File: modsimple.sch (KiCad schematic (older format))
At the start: 13 parts, among them J1 MICROUSB, P1 CONN_10, Q2 FDD8870, U1 MAX1555

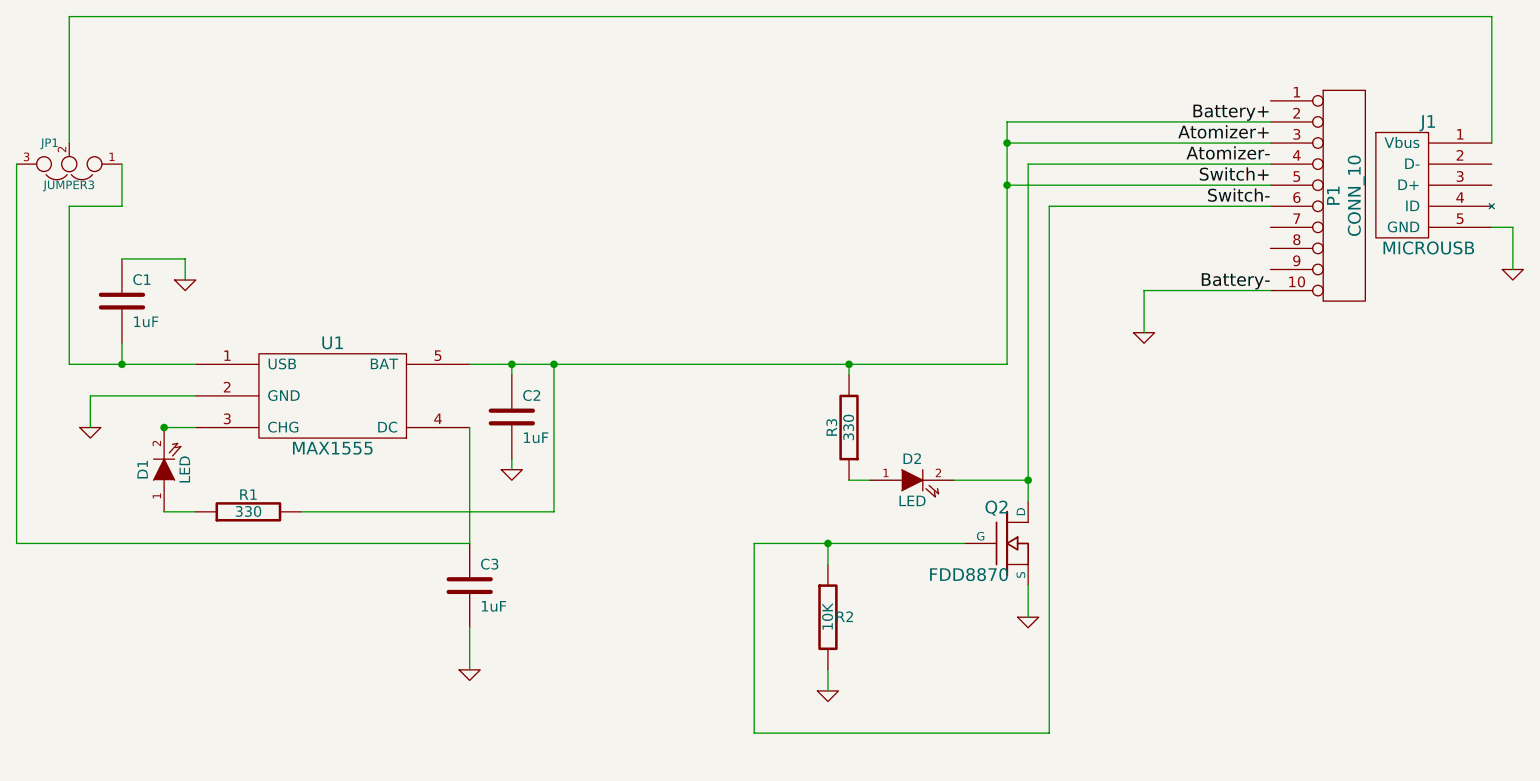
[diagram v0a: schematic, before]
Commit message: cleanup
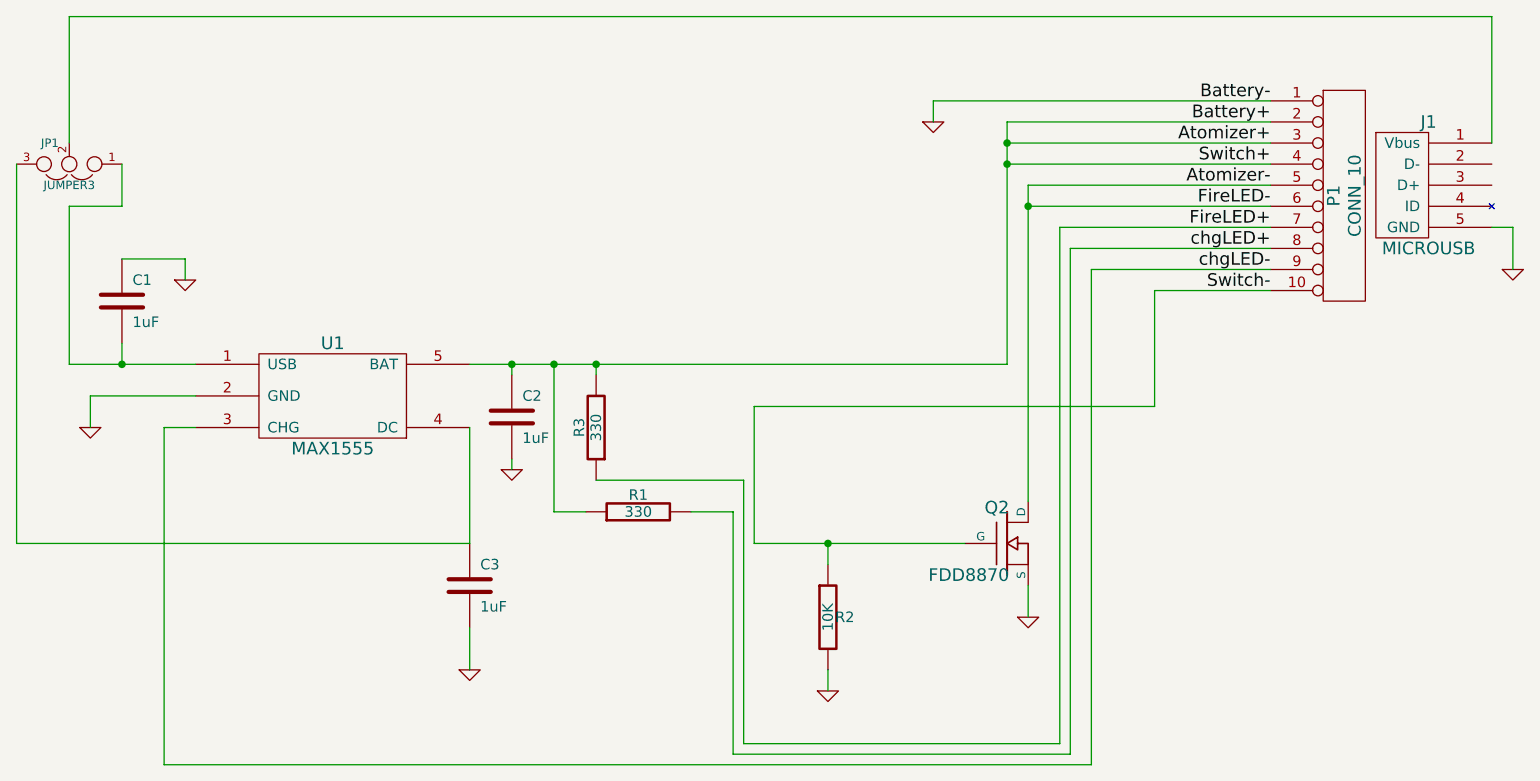
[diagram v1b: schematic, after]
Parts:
- removed D1, D2: LED, symbol LED
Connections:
- net Atomizer+: now also P1.4 (P4), R1.1; no longer P1.5 (P5), R1.2
- net Atomizer-: now also P1.5 (P5), P1.6 (P6); no longer P1.4 (P4)
- net GND: now also P1.1 (P1); no longer P1.10 (P10)
- net Switch-: now also P1.10 (P10); no longer P1.6 (P6)
- net FireLED+: now reaches P1.7 (P7)
- net FireLED+: now also R3.1
- net chgLED+: now reaches P1.8 (P8)
- net chgLED+: now also R1.2
- net chgLED-: now reaches P1.9 (P9)
- net chgLED-: now also U1.3 (CHG)
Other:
- moved on the sheet: R1, R3
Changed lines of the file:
@@
-EESchema Schematic File Version 2  date Mon 04 Mar 2013 02:49:37 AM CST
+EESchema Schematic File Version 2  date Tue 12 Mar 2013 12:01:35 PM CDT
 LIBS:power
 LIBS:device
@@
 LIBS:mod
 LIBS:modsimple-cache
-EELAYER 25  0
+EELAYER 27 0
 EELAYER END
-$Descr A4 11700 8267
+$Descr A4 11693 8268
 encoding utf-8
 Sheet 1 1
 Title ""
-Date "3 mar 2013"
+Date "12 mar 2013"
 Rev ""
 Comp ""
@@
 Comment4 ""
 $EndDescr
-Wire Wire Line
-	9450 4100 9450 3900
-Wire Wire Line
-	9450 3900 10050 3900
-Wire Wire Line
-	10050 3100 8800 3100
-Connection ~ 8050 4250
-Wire Wire Line
-	8050 4300 8050 4250
-Wire Wire Line
-	8600 5100 7600 5100
-Wire Wire Line
-	7600 5100 7600 6000
-Wire Wire Line
-	7600 6000 9000 6000
-Wire Wire Line
-	6250 4250 8800 4250
-Wire Wire Line
-	8800 4250 8800 3100
-Wire Wire Line
-	4350 2600 11100 2600
-Wire Wire Line
-	4350 2600 4350 3200
-Connection ~ 7950 5100
-Wire Wire Line
-	7950 5100 7950 5200
-Wire Wire Line
-	8900 5300 8900 5450
-Wire Wire Line
-	6250 4550 6250 5100
-Wire Wire Line
-	6250 5100 4100 5100
-Wire Wire Line
-	4100 5100 4100 3300
-Wire Wire Line
-	6450 4700 6450 4750
-Connection ~ 4600 4250
-Wire Wire Line
-	4600 4150 4600 4250
-Wire Wire Line
-	4950 4250 4350 4250
-Wire Wire Line
-	11100 2600 11100 3200
-Connection ~ 6650 4250
-Wire Wire Line
-	4950 4400 4450 4400
-Wire Wire Line
-	4450 4400 4450 4550
-Connection ~ 4800 4550
-Wire Wire Line
-	4600 3750 4900 3750
-Wire Wire Line
-	4900 3750 4900 3850
-Wire Wire Line
-	6450 4300 6450 4250
-Connection ~ 6450 4250
-Wire Wire Line
-	4800 4550 4950 4550
-Wire Wire Line
-	6650 4250 6650 4950
-Wire Wire Line
-	4600 3300 4600 3500
-Wire Wire Line
-	4600 3500 4350 3500
-Wire Wire Line
-	4350 3500 4350 4250
-Wire Wire Line
-	11100 3600 11200 3600
-Wire Wire Line
-	11200 3600 11200 3800
-Wire Wire Line
-	10050 3300 8900 3300
-Wire Wire Line
-	8900 3300 8900 4900
-Wire Wire Line
-	10050 3500 9000 3500
-Wire Wire Line
-	9000 3500 9000 6000
-Wire Wire Line
-	7950 5700 7950 5800
-Wire Wire Line
-	8800 3200 10050 3200
-Connection ~ 8800 3200
-Wire Wire Line
-	6250 5500 6250 5700
-Wire Wire Line
-	6650 4950 5450 4950
-Wire Wire Line
-	4800 4950 4950 4950
-Wire Wire Line
-	8050 4800 8150 4800
-Wire Wire Line
-	8550 4800 8900 4800
-Connection ~ 8900 4800
-Wire Wire Line
-	10050 3400 8800 3400
-Connection ~ 8800 3400
 $Comp
 L R R3
 U 1 1 5133879A
-P 8050 4550
-F 0 "R3" V 8130 4550 50  0000 C CNN
-F 1 "330" V 8050 4550 50  0000 C CNN
-	1    8050 4550
+P 6850 4550
+F 0 "R3" V 6930 4550 50  0000 C CNN
+F 1 "330" V 6850 4550 50  0000 C CNN
+F 2 "" H 6850 4550 60  0001 C CNN
+F 3 "" H 6850 4550 60  0001 C CNN
+	1    6850 4550
 	-1   0    0    1
-$EndComp
-$Comp
-L LED D2
-U 1 1 51338773
-P 8350 4800
-F 0 "D2" H 8350 4900 50  0000 C CNN
-F 1 "LED" H 8350 4700 50  0000 C CNN
-	1    8350 4800
-	1    0    0    -1
-$EndComp
-$Comp
-L LED D1
-U 1 1 512B1B1D
-P 4800 4750
-F 0 "D1" H 4800 4850 50  0000 C CNN
-F 1 "LED" H 4800 4650 50  0000 C CNN
-	1    4800 4750
-	0    -1   -1   0
 $EndComp
 $Comp
@@
 F 0 "#PWR01" H 6250 5700 30  0001 C CNN
 F 1 "GND" H 6250 5630 30  0001 C CNN
+F 2 "" H 6250 5700 60  0001 C CNN
+F 3 "" H 6250 5700 60  0001 C CNN
 	1    6250 5700
 	1    0    0    -1
@@
 F 0 "C3" H 6300 5400 50  0000 L CNN
 F 1 "1uF" H 6300 5200 50  0000 L CNN
+F 2 "" H 6250 5300 60  0001 C CNN
+F 3 "" H 6250 5300 60  0001 C CNN
 	1    6250 5300
 	1    0    0    -1
@@
 F 0 "#PWR02" H 7950 5800 30  0001 C CNN
 F 1 "GND" H 7950 5730 30  0001 C CNN
+F 2 "" H 7950 5800 60  0001 C CNN
+F 3 "" H 7950 5800 60  0001 C CNN
 	1    7950 5800
 	1    0    0    -1
@@
 F 0 "R2" H 8030 5450 50  0000 C CNN
 F 1 "10K" V 7950 5450 50  0000 C CNN
+F 2 "" H 7950 5450 60  0001 C CNN
+F 3 "" H 7950 5450 60  0001 C CNN
 	1    7950 5450
 	1    0    0    -1
 $EndComp
-Text Label 10050 3500 2    60   ~ 0
+Text Label 10050 3900 2    60   ~ 0
 Switch-
+Text Label 10050 3300 2    60   ~ 0
+Switch+
 Text Label 10050 3400 2    60   ~ 0
-Switch+
-Text Label 10050 3300 2    60   ~ 0
 Atomizer-
 $Comp
@@
 F 0 "#PWR03" H 8900 5450 30  0001 C CNN
 F 1 "GND" H 8900 5380 30  0001 C CNN
+F 2 "" H 8900 5450 60  0001 C CNN
+F 3 "" H 8900 5450 60  0001 C CNN
 	1    8900 5450
 	1    0    0    -1
@@
 F 0 "Q2" H 8810 5270 60  0000 R CNN
 F 1 "FDD8870" H 8810 4950 60  0000 R CNN
+F 2 "" H 8800 5100 60  0001 C CNN
+F 3 "" H 8800 5100 60  0001 C CNN
 	1    8800 5100
 	1    0    0    -1
@@
 Text Label 10050 3200 2    60   ~ 0
 Atomizer+
-Text Label 10050 3900 2    60   ~ 0
+Text Label 10050 3000 2    60   ~ 0
 Battery-
 Text Label 10050 3100 2    60   ~ 0
@@
 F 0 "#PWR04" H 11200 3800 30  0001 C CNN
 F 1 "GND" H 11200 3730 30  0001 C CNN
+F 2 "" H 11200 3800 60  0001 C CNN
+F 3 "" H 11200 3800 60  0001 C CNN
 	1    11200 3800
 	1    0    0    -1
@@
 F 0 "JP1" H 4400 3200 40  0000 L CNN
 F 1 "JUMPER3" H 4350 3400 40  0000 C CNN
+F 2 "" H 4350 3300 60  0001 C CNN
+F 3 "" H 4350 3300 60  0001 C CNN
 	1    4350 3300
 	-1   0    0    1
@@
 F 0 "#PWR05" H 6450 4750 30  0001 C CNN
 F 1 "GND" H 6450 4680 30  0001 C CNN
+F 2 "" H 6450 4750 60  0001 C CNN
+F 3 "" H 6450 4750 60  0001 C CNN
 	1    6450 4750
 	1    0    0    -1
@@
 F 0 "C2" H 6500 4600 50  0000 L CNN
 F 1 "1uF" H 6500 4400 50  0000 L CNN
+F 2 "" H 6450 4500 60  0001 C CNN
+F 3 "" H 6450 4500 60  0001 C CNN
 	1    6450 4500
 	1    0    0    -1
@@
 F 0 "#PWR06" H 4900 3850 30  0001 C CNN
 F 1 "GND" H 4900 3780 30  0001 C CNN
+F 2 "" H 4900 3850 60  0001 C CNN
+F 3 "" H 4900 3850 60  0001 C CNN
 	1    4900 3850
 	1    0    0    -1
@@
 F 0 "C1" H 4650 4050 50  0000 L CNN
 F 1 "1uF" H 4650 3850 50  0000 L CNN
+F 2 "" H 4600 3950 60  0001 C CNN
+F 3 "" H 4600 3950 60  0001 C CNN
 	1    4600 3950
 	1    0    0    -1
@@
 L R R1
 U 1 1 512B94C6
-P 5200 4950
-F 0 "R1" V 5280 4950 50  0000 C CNN
-F 1 "330" V 5200 4950 50  0000 C CNN
-	1    5200 4950
+P 7050 4950
+F 0 "R1" V 7130 4950 50  0000 C CNN
+F 1 "330" V 7050 4950 50  0000 C CNN
+F 2 "" H 7050 4950 60  0001 C CNN
+F 3 "" H 7050 4950 60  0001 C CNN
+	1    7050 4950
 	0    -1   -1   0
 $EndComp
@@
 F 0 "#PWR07" H 4450 4550 30  0001 C CNN
 F 1 "GND" H 4450 4480 30  0001 C CNN
+F 2 "" H 4450 4550 60  0001 C CNN
+F 3 "" H 4450 4550 60  0001 C CNN
 	1    4450 4550
 	1    0    0    -1
@@
 F 0 "J1" H 10800 4300 60  0000 C CNN
 F 1 "MICROUSB" H 10800 3700 60  0000 C CNN
+F 2 "" H 10800 3700 60  0001 C CNN
+F 3 "" H 10800 3700 60  0001 C CNN
 	1    10800 3700
 	1    0    0    -1
@@
 F 0 "U1" H 5600 5150 60  0000 C CNN
 F 1 "MAX1555" H 5600 4650 60  0000 C CNN
+F 2 "" H 5600 4650 60  0001 C CNN
+F 3 "" H 5600 4650 60  0001 C CNN
 	1    5600 4650
 	1    0    0    -1
@@
 L GND #PWR08
 U 1 1 512AF9E3
-P 9450 4100
-F 0 "#PWR08" H 9450 4100 30  0001 C CNN
-F 1 "GND" H 9450 4030 30  0001 C CNN
-	1    9450 4100
+P 8450 3100
+F 0 "#PWR08" H 8450 3100 30  0001 C CNN
+F 1 "GND" H 8450 3030 30  0001 C CNN
+F 2 "" H 8450 3100 60  0001 C CNN
+F 3 "" H 8450 3100 60  0001 C CNN
+	1    8450 3100
 	1    0    0    -1
 $EndComp
@@
 F 0 "P1" V 10350 3450 60  0000 C CNN
 F 1 "CONN_10" V 10450 3450 60  0000 C CNN
+F 2 "" H 10400 3450 60  0001 C CNN
+F 3 "" H 10400 3450 60  0001 C CNN
 	1    10400 3450
 	1    0    0    -1
 $EndComp
+Text Label 10050 3600 2    60   ~ 0
+FireLED+
+Text Label 10050 3700 2    60   ~ 0
+chgLED+
+Text Label 10050 3800 2    60   ~ 0
+chgLED-
+Text Label 10050 3500 2    60   ~ 0
+FireLED-
+Wire Wire Line
+	8450 3100 8450 3000
+Wire Wire Line
+	8450 3000 10050 3000
+Wire Wire Line
+	10050 3100 8800 3100
+Connection ~ 6850 4250
+Wire Wire Line
+	6850 4250 6850 4300
+Wire Wire Line
+	7600 5100 8600 5100
+Wire Wire Line
+	8800 4250 6250 4250
+Wire Wire Line
+	8800 3100 8800 4250
+Wire Wire Line
+	4350 2600 11100 2600
+Wire Wire Line
+	4350 2600 4350 3200
+Connection ~ 7950 5100
+Wire Wire Line
+	7950 5100 7950 5200
+Wire Wire Line
+	8900 5300 8900 5450
+Wire Wire Line
+	6250 4550 6250 5100
+Wire Wire Line
+	6250 5100 4100 5100
+Wire Wire Line
+	4100 5100 4100 3300
+Wire Wire Line
+	6450 4700 6450 4750
+Connection ~ 4600 4250
+Wire Wire Line
+	4600 4150 4600 4250
+Wire Wire Line
+	4350 4250 4950 4250
+Wire Wire Line
+	11100 2600 11100 3200
+Connection ~ 6650 4250
+Wire Wire Line
+	4950 4400 4450 4400
+Wire Wire Line
+	4450 4400 4450 4550
+Wire Wire Line
+	4600 3750 4900 3750
+Wire Wire Line
+	4900 3750 4900 3850
+Wire Wire Line
+	6450 4300 6450 4250
+Connection ~ 6450 4250
+Wire Wire Line
+	6650 4250 6650 4950
+Wire Wire Line
+	4600 3300 4600 3500
+Wire Wire Line
+	4600 3500 4350 3500
+Wire Wire Line
+	4350 3500 4350 4250
+Wire Wire Line
+	11100 3600 11200 3600
+Wire Wire Line
+	11200 3600 11200 3800
+Wire Wire Line
+	8900 3400 8900 4900
+Wire Wire Line
+	7950 5700 7950 5800
+Wire Wire Line
+	8800 3200 10050 3200
+Connection ~ 8800 3200
+Wire Wire Line
+	6250 5500 6250 5700
+Connection ~ 8800 3300
+Wire Wire Line
+	6650 4950 6800 4950
+Wire Wire Line
+	6850 4800 7550 4800
+Wire Wire Line
+	7550 4800 7550 6050
+Wire Wire Line
+	7550 6050 9050 6050
+Wire Wire Line
+	9050 6050 9050 3600
+Wire Wire Line
+	9050 3600 10050 3600
+Wire Wire Line
+	7300 4950 7500 4950
+Wire Wire Line
+	7500 4950 7500 6100
+Wire Wire Line
+	7500 6100 9100 6100
+Wire Wire Line
+	9100 6100 9100 3700
+Wire Wire Line
+	9100 3700 10050 3700
+Wire Wire Line
+	10050 3800 9200 3800
+Wire Wire Line
+	9200 3800 9200 6150
+Wire Wire Line
+	9200 6150 4800 6150
+Wire Wire Line
+	4800 6150 4800 4550
+Wire Wire Line
+	4800 4550 4950 4550
+Wire Wire Line
+	10050 3300 8800 3300
+Wire Wire Line
+	8900 3400 10050 3400
+Wire Wire Line
+	10050 3900 9500 3900
+Wire Wire Line
+	9500 3900 9500 4450
+Wire Wire Line
+	9500 4450 7600 4450
+Wire Wire Line
+	7600 4450 7600 5100
+Wire Wire Line
+	10050 3500 8900 3500
+Connection ~ 8900 3500
 $EndSCHEMATC
